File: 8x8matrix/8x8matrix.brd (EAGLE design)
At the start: 60.4 x 60.5 mm, 5 parts, among them IC1 74595

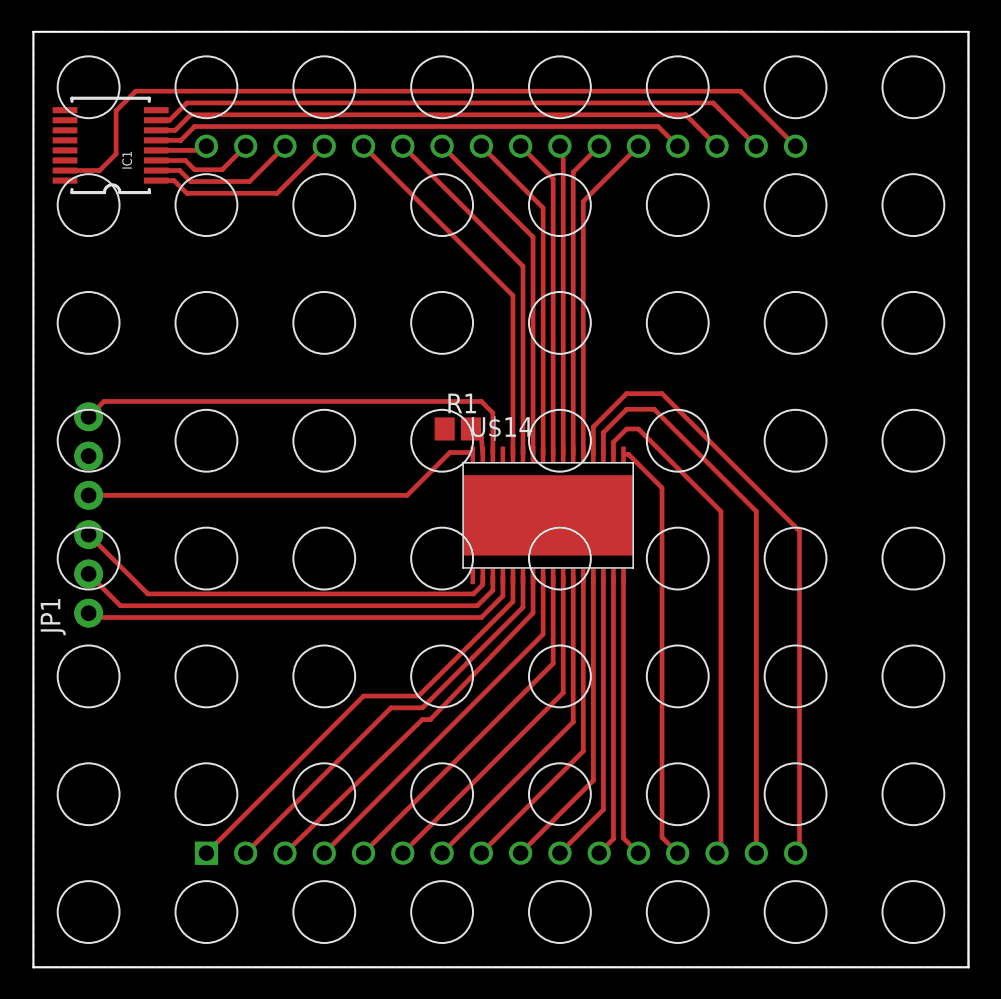
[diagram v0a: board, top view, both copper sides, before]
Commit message: tlc3
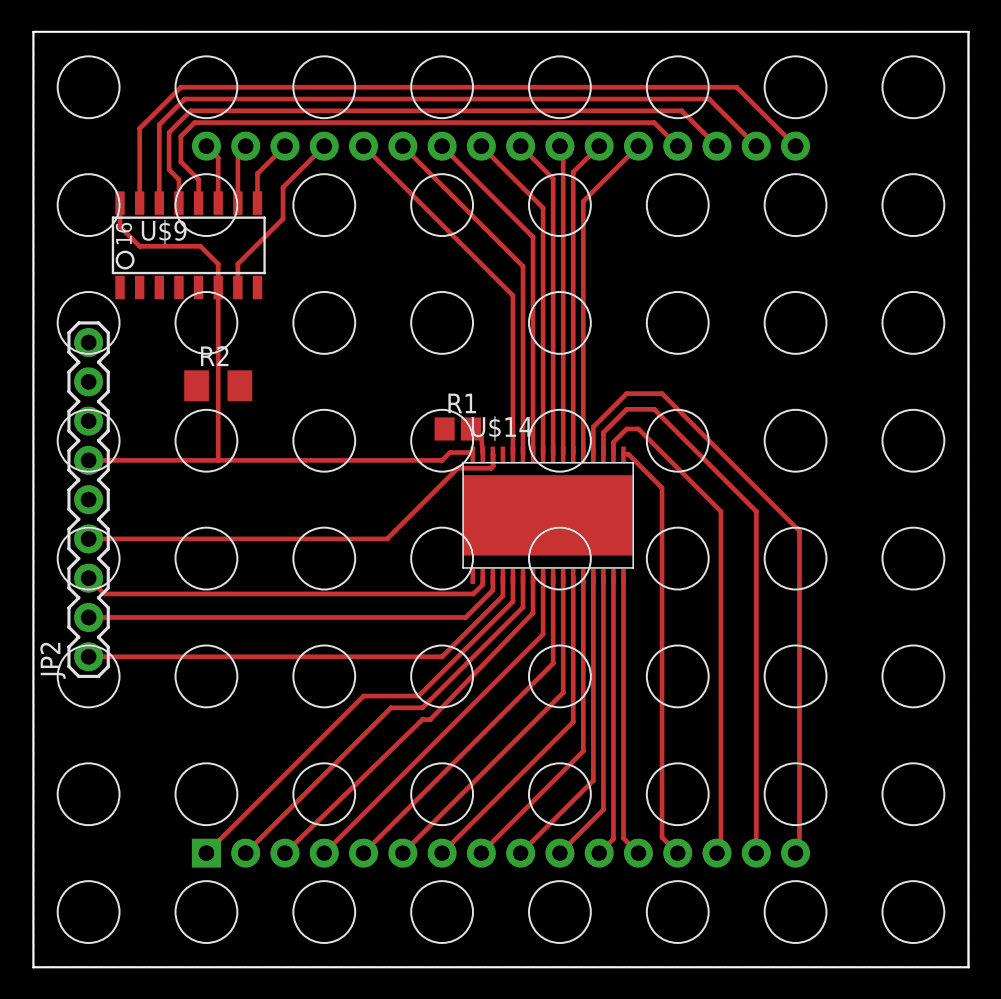
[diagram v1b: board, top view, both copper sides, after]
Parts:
- removed IC1: 74595, SparkFun-DigitalIC:TSSOP16
- removed JP1: (no value), SparkFun-Connectors:1X06
- added JP2: M09, SparkFun-Connectors:1X09
- added R2: 0R, resistor:M1206
- added U$9: CD74HC238M, mylib:SO-16
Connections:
- removed net XLAT: JP1.6, U$14.30
- new net N$35: U$1.P29, U$9.7
- net 5.0V: now also JP2.6, U$9.16, U$9.6; no longer IC1.16, JP1.4
- net BLANK: now also JP2.3; no longer JP1.3
- net GND: now also JP2.5, R2.1, R2.2, U$9.4, U$9.5, U$9.8; no longer IC1.8, JP1.5
- net N$25: now also JP2.4, U$14.30; no longer IC1.1, U$1.P29
- net N$26: now also U$9.9; no longer IC1.2
- net N$28: now also JP2.2; no longer JP1.2
- net N$29: now also U$9.10; no longer IC1.3
- net N$30: now also U$9.11; no longer IC1.4
- net N$31: now also U$9.12; no longer IC1.5
- net N$32: now also U$9.13; no longer IC1.6
- net N$33: now also U$9.14; no longer IC1.7
- net N$34: now also U$9.15; no longer IC1.15
- net SIN: now also JP2.1; no longer JP1.1
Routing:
- net XLAT: track 29.5 -> 0.00 mm
- net 5.0V: track 26.0 -> 46.7 mm
- net N$25: track 12.5 -> 28.9 mm
- net N$35: track 0.00 -> 11.5 mm
- net N$33: track 40.4 -> 45.6 mm
- net N$26: track 9.57 -> 4.42 mm
- net N$32: track 37.5 -> 41.8 mm
- net N$31: track 34.6 -> 37.9 mm
- net N$29: track 6.67 -> 3.89 mm
- net N$34: track 52.5 -> 49.9 mm
- net BLANK: track 27.9 -> 26.7 mm
- net SIN: track 28.7 -> 29.7 mm
- net N$30: track 3.36 -> 4.00 mm
- net N$28: track 28.3 -> 27.8 mm
